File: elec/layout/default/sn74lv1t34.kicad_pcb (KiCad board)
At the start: 2 copper layers, 225.7 x 100.8 mm, 0 parts

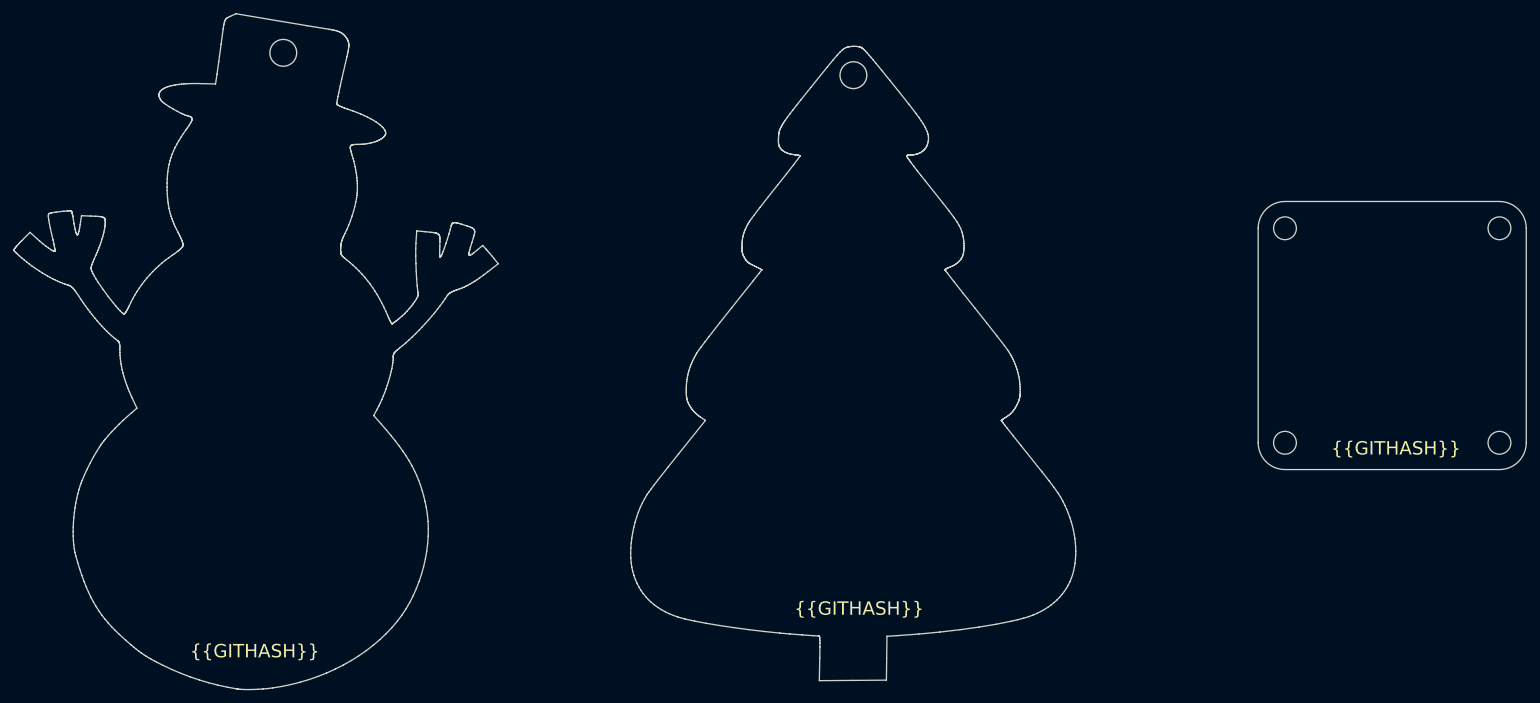
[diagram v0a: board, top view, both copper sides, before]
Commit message: added layout
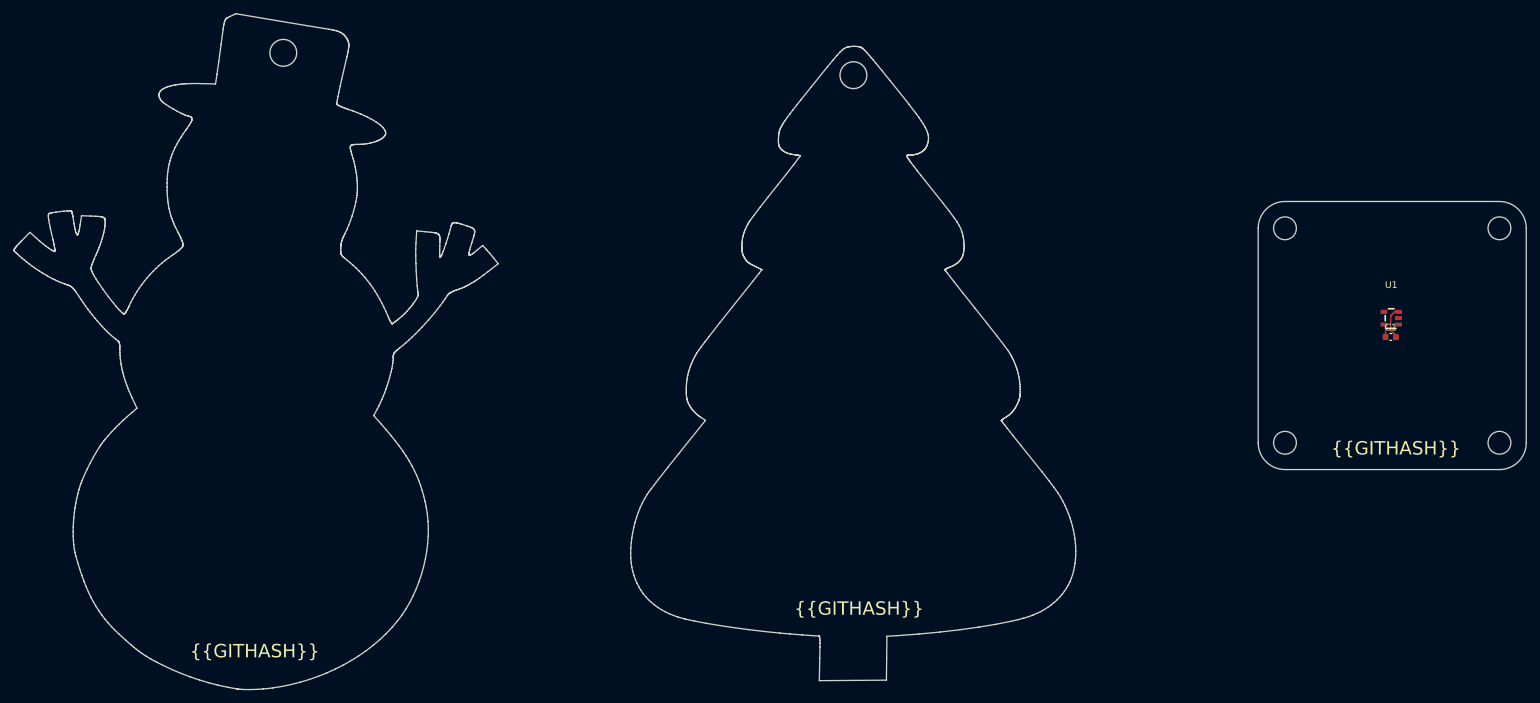
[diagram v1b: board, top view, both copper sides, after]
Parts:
- added C1: 50V 100nF X7R ±10% 0603 Multilayer Ceramic Capacitors MLCC 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, lib:C0603, F.Cu at (241.4, 98.0)
- added U1: , lib:SOT-23-5_L2.9-W1.6-P0.95-LS2.8-BR, F.Cu at (241.5, 95.2)
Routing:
- net gnd: track 0.00 -> 4.91 mm
- net vcc: track 0.00 -> 1.97 mm
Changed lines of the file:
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@@
   )
   (net 0 "")
+  (net 1 "input")
+  (net 2 "gnd")
+  (net 3 "nc")
+  (net 4 "output")
+  (net 5 "vcc")
+  (footprint "lib:C0603" (layer "F.Cu")
+    (at 241.4 98)
+    (descr "Capacitor SMD 0603 (1608 Metric), square (rectangular) end terminal, IPC_7351 nominal, (Body size source: IPC-SM-782 page 76, https://www.pcb-3d.com/wordpress/wp-content/uploads/ipc-sm-782a_amendment_1_and_2.pdf), generated with kicad-footprint-generator")
+    (tags "capacitor")
+    (attr smd)
+    (fp_text reference "C1" (at 0 -1.43) (layer "F.SilkS")
+        (effects (font (size 1 1) (thickness 0.15)))
+    )
+    (fp_text value "50V 100nF X7R ±10% 0603  Multilayer Ceramic Capacitors MLCC - SMD/SMT ROHS" (at 0 1.43) (layer "F.Fab")
+        (effects (font (size 1 1) (thickness 0.15)))
+    )
+    (fp_text user "${REFERENCE}" (at 0 0) (layer "F.Fab")
+        (effects (font (size 0.4 0.4) (thickness 0.06)))
+    )
+    (fp_line (start -0.14058 -0.51) (end 0.14058 -0.51)
+      (stroke (width 0.12) (type solid)) (layer "F.SilkS"))
+    (fp_line (start -0.14058 0.51) (end 0.14058 0.51)
+      (stroke (width 0.12) (type solid)) (layer "F.SilkS"))
+    (fp_line (start -1.48 -0.73) (end 1.48 -0.73)
+      (stroke (width 0.05) (type solid)) (layer "F.CrtYd"))
+    (fp_line (start -1.48 0.73) (end -1.48 -0.73)
+      (stroke (width 0.05) (type solid)) (layer "F.CrtYd"))
+    (fp_line (start 1.48 -0.73) (end 1.48 0.73)
+      (stroke (width 0.05) (type solid)) (layer "F.CrtYd"))
+    (fp_line (start 1.48 0.73) (end -1.48 0.73)
+      (stroke (width 0.05) (type solid)) (layer "F.CrtYd"))
+    (fp_line (start -0.8 -0.4) (end 0.8 -0.4)
+      (stroke (width 0.1) (type solid)) (layer "F.Fab"))
+    (fp_line (start -0.8 0.4) (end -0.8 -0.4)
+      (stroke (width 0.1) (type solid)) (layer "F.Fab"))
+    (fp_line (start 0.8 -0.4) (end 0.8 0.4)
+      (stroke (width 0.1) (type solid)) (layer "F.Fab"))
+    (fp_line (start 0.8 0.4) (end -0.8 0.4)
+      (stroke (width 0.1) (type solid)) (layer "F.Fab"))
+    (pad "1" smd roundrect (at -0.775 0) (size 0.9 0.95) (layers "F.Cu" "F.Paste" "F.Mask") (roundrect_rratio 0.25)
+      (net 5 "vcc") (pintype "stereo"))
+    (pad "2" smd roundrect (at 0.775 0) (size 0.9 0.95) (layers "F.Cu" "F.Paste" "F.Mask") (roundrect_rratio 0.25)
+      (net 2 "gnd") (pintype "stereo"))
+    (model "${KICAD6_3DMODEL_DIR}/Capacitor_SMD.3dshapes/C_0603_1608Metric.wrl"
+      (offset (xyz 0 0 0))
+      (scale (xyz 1 1 1))
+      (rotate (xyz 0 0 0))
+    )
+  )
+  (footprint "lib:SOT-23-5_L2.9-W1.6-P0.95-LS2.8-BR" (layer "F.Cu")
+    (at 241.47 95.19)
+    (attr smd)
+    (fp_text reference "U1" (at 0 -4.95) (layer "F.SilkS")
+        (effects (font (size 1 1) (thickness 0.15)))
+    )
+    (fp_text value "" (at 0 4.95) (layer "F.Fab")
+        (effects (font (size 1 1) (thickness 0.15)))
+    )
+    (fp_text user "${REFERENCE}" (at 0 0) (layer "F.Fab")
+        (effects (font (size 1 1) (thickness 0.15)))
+    )
+    (fp_line (start -0.89 0.38) (end -0.89 -0.38)
+      (stroke (width 0.25) (type solid)) (layer "F.SilkS"))
+    (fp_line (start -0.7 1.53) (end 0.7 1.53)
+      (stroke (width 0.25) (type solid)) (layer "F.SilkS"))
+    (fp_line (start -0.42 -1.39) (end 0.42 -1.39)
+      (stroke (width 0.25) (type solid)) (layer "F.SilkS"))
+    (fp_circle (center 1.11 1.25) (end 1.26 1.25)
+      (stroke (width 0.3) (type solid)) (fill none) (layer "Cmts.User"))
+    (fp_circle (center 1.4 1.45) (end 1.43 1.45)
+      (stroke (width 0.06) (type solid)) (fill none) (layer "F.Fab"))
+    (pad "1" smd rect (at 1.1 0.95 90) (size 0.6 1) (layers "F.Cu" "F.Paste" "F.Mask")
+      (net 3 "nc") (pintype "stereo"))
+    (pad "2" smd rect (at 1.1 0 90) (size 0.6 1) (layers "F.Cu" "F.Paste" "F.Mask")
+      (net 1 "input") (pintype "stereo"))
+    (pad "3" smd rect (at 1.1 -0.95 90) (size 0.6 1) (layers "F.Cu" "F.Paste" "F.Mask")
+      (net 2 "gnd") (pintype "stereo"))
+    (pad "4" smd rect (at -1.1 -0.95 90) (size 0.6 1) (layers "F.Cu" "F.Paste" "F.Mask")
+      (net 4 "output") (pintype "stereo"))
+    (pad "5" smd rect (at -1.1 0.95 90) (size 0.6 1) (layers "F.Cu" "F.Paste" "F.Mask")
+      (net 5 "vcc") (pintype "stereo"))
+    (model "/Users/nickk/projects/chess-clock/.ato/modules/smart-knob/.ato/modules/sn74lv1t34/elec/footprints/footprints.3dshapes/SOT-23-5_L2.9-W1.6-P0.95-LS2.8-BR.wrl"
+      (offset (xyz 0 -0 -0))
+      (scale (xyz 1 1 1))
+      (rotate (xyz 0 0 270))
+    )
+  )
   (gr_circle (center 225.62 81.79) (end 227.32 81.79)
     (stroke (width 0.1) (type solid)) (fill none) (layer "Edge.Cuts"))
@@
       (xy 69.100734 49.778315)
     )
-    (stroke (width 0) (type solid)) (fill none) (layer "Edge.Cuts"))
+    (stroke (width 0.1) (type solid)) (fill none) (layer "Edge.Cuts"))
   (gr_arc (start 261.62 113.79) (mid 260.448427 116.618427) (end 257.62 117.79)
     (stroke (width 0.1) (type solid)) (layer "Edge.Cuts"))
@@
     (effects (font (size 2 2) (thickness 0.1)) (justify left bottom))
   )
+  (segment (start 242.57 94.24) (end 241.99 94.24) (width 0.25) (layer "F.Cu") (net 2))
+  (segment (start 242.175 97.775) (end 242.175 98) (width 0.25) (layer "F.Cu") (net 2))
+  (segment (start 241.99 94.24) (end 241.4 94.83) (width 0.25) (layer "F.Cu") (net 2))
+  (segment (start 241.4 97) (end 242.175 97.775) (width 0.25) (layer "F.Cu") (net 2))
+  (segment (start 241.4 94.83) (end 241.4 97) (width 0.25) (layer "F.Cu") (net 2))
+  (segment (start 240.625 96.395) (end 240.37 96.14) (width 0.25) (layer "F.Cu") (net 5))
+  (segment (start 240.625 98) (end 240.625 96.395) (width 0.25) (layer "F.Cu") (net 5))
   (group "" (id 6c1ef9f7-0f34-47bb-ac1a-76df23fb396e)
     (members
